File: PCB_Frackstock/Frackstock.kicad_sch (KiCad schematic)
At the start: 0 parts

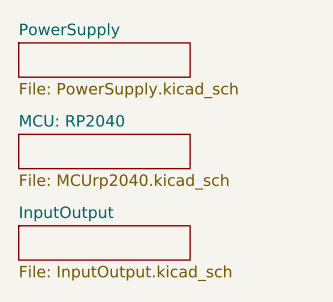
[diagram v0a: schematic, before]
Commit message: Schema_fertig
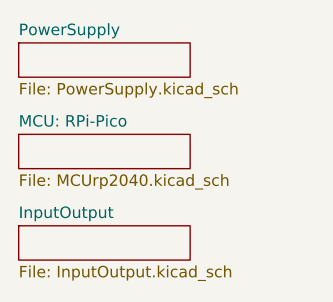
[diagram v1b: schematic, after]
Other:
- sheet MCU: RP2040 renamed MCU: RPi-Pico
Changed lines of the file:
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@@
     (stroke (width 0.1524) (type solid))
     (fill (color 0 0 0 0.0000))
-    (property "Sheetname" "MCU: RP2040" (at 22.86 31.0384 0)
+    (property "Sheetname" "MCU: RPi-Pico" (at 22.86 31.0384 0)
       (effects (font (size 1.27 1.27)) (justify left bottom))
     )

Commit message: Schema-review-1
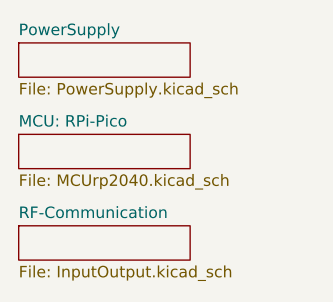
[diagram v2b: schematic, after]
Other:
- sheet InputOutput renamed RF-Communication
- company: (none) -> Eberkreis
- title: (none) -> Frackstock ET2024
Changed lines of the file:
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@@
 (kicad_sch (version 20230121) (generator eeschema)
   (paper "A4")
+  (title_block
+    (title "Frackstock ET2024")
+    (date "2024-03-24")
+    (rev "2")
+    (company "Eberkreis")
+  )
   (sheet (at 22.86 41.91) (size 19.05 3.81) (fields_autoplaced)
     (stroke (width 0.1524) (type solid))
     (fill (color 0 0 0 0.0000))
-    (property "Sheetname" "InputOutput" (at 22.86 41.1984 0)
+    (property "Sheetname" "RF-Communication" (at 22.86 41.1984 0)
       (effects (font (size 1.27 1.27)) (justify left bottom))
     )

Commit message: Fracstock PCB final commit
DRC check, PCB review done, ready to order
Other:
- company: Eberkreis -> Eberkreis Engineering
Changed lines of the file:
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@@
     (date "2024-03-24")
     (rev "2")
-    (company "Eberkreis")
+    (company "Eberkreis Engineering")
   )
   (sheet (at 22.86 41.91) (size 19.05 3.81) (fields_autoplaced)
